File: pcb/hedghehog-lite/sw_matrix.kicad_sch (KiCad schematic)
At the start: 8 parts, among them K00 1u, K01 1u, K10 1u, K11 1u

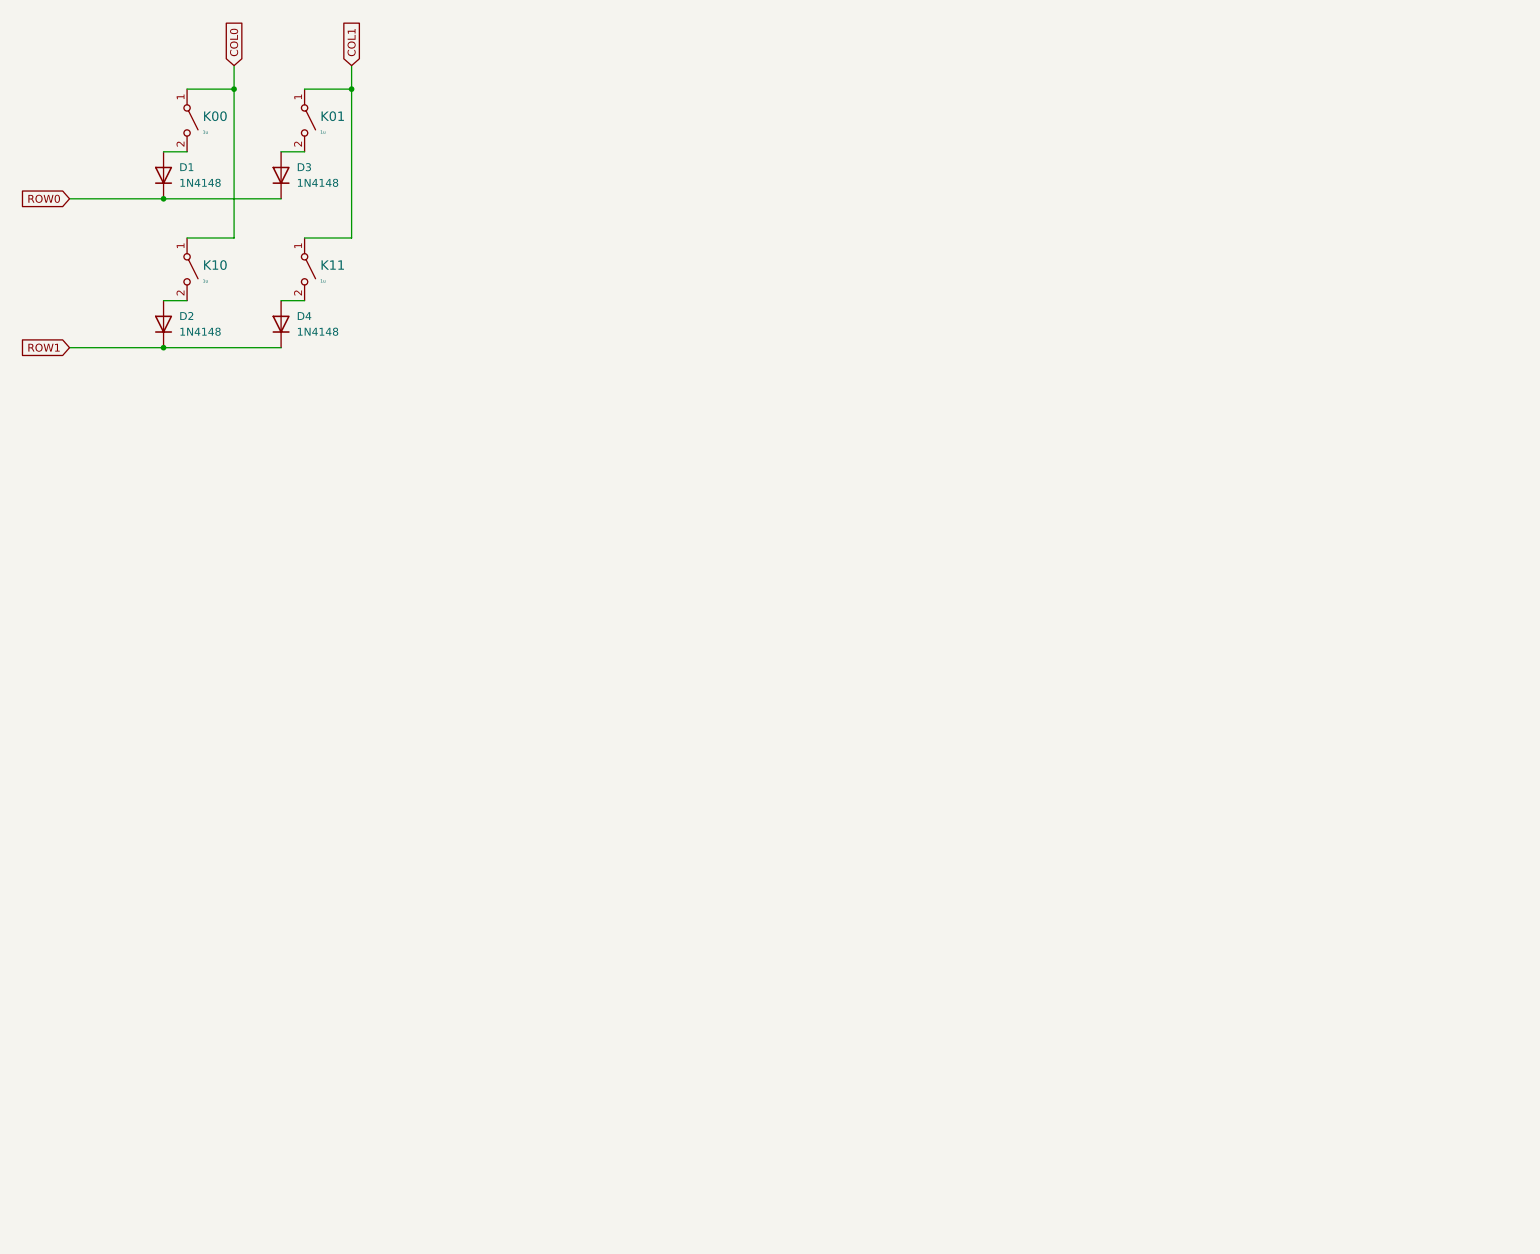
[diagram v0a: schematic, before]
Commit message: More edits to the schematic building v1
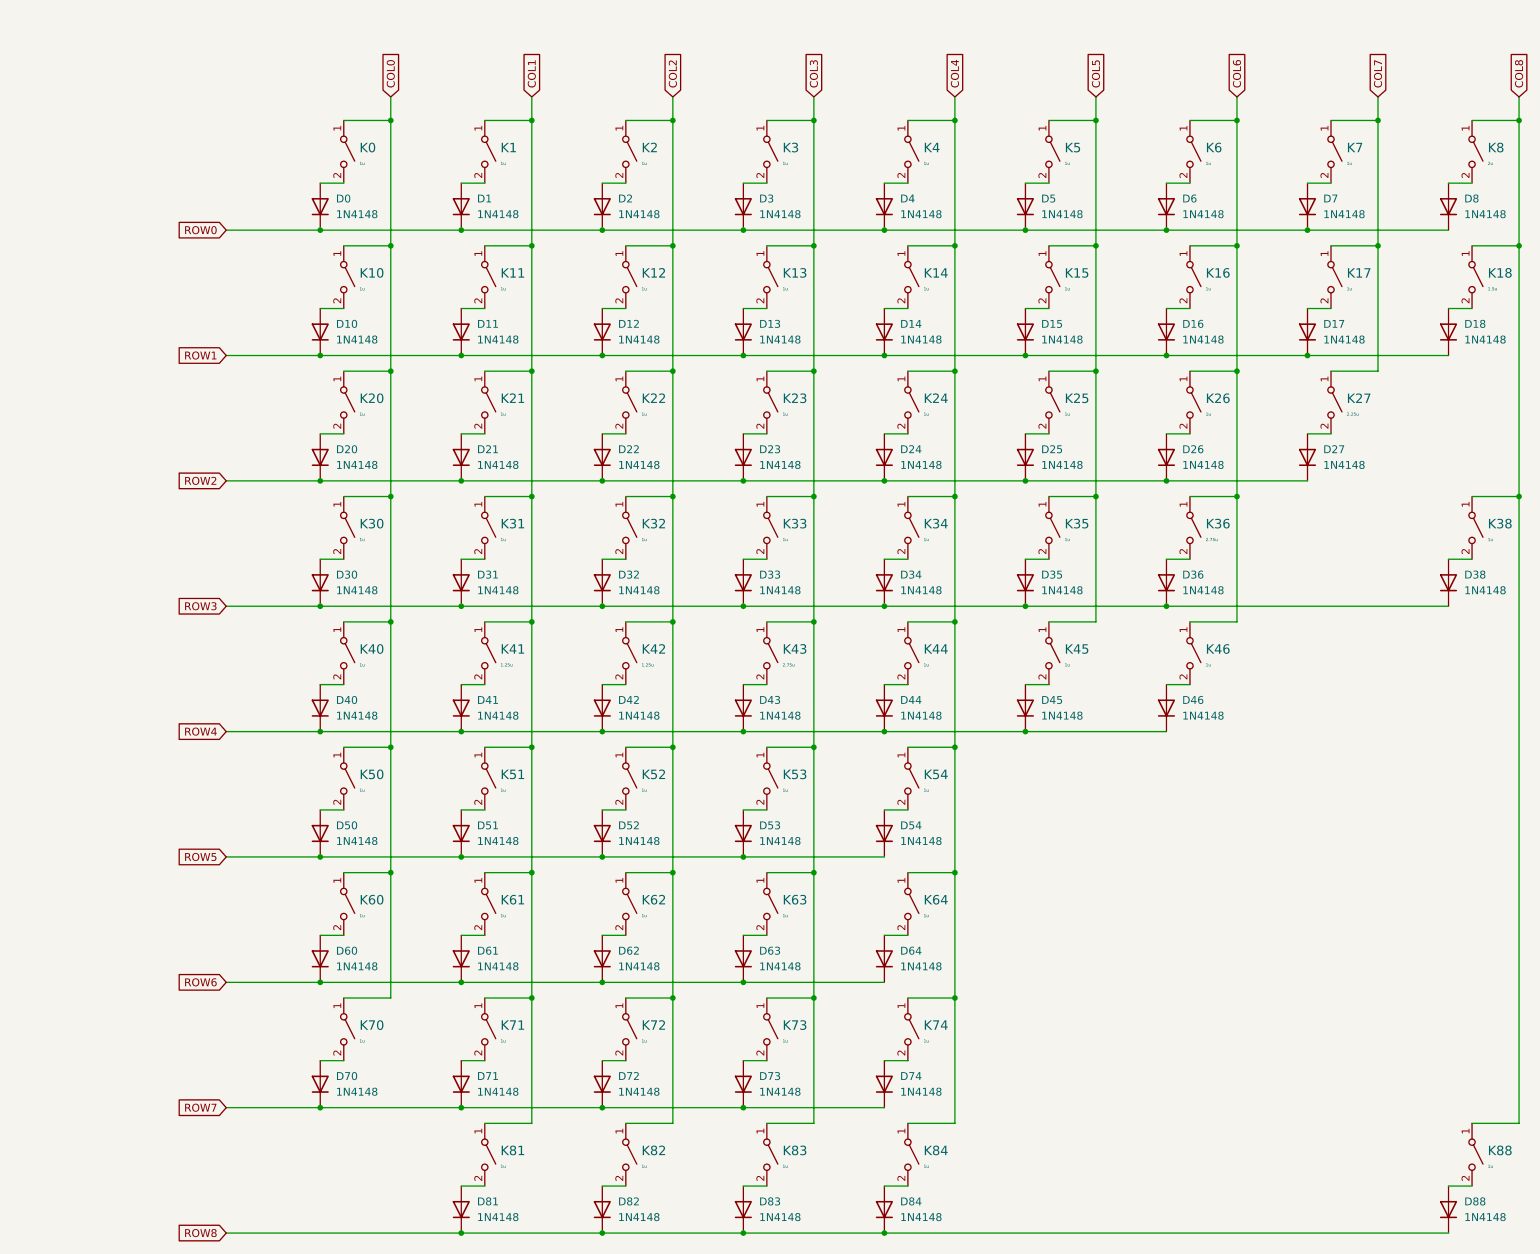
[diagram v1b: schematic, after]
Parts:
- added D12, D13, D14, D15, D16, D17, D18, D2, D3, D4, D5, D6, D7, D70, D8, D81: 1N4148, Diode_SMD:D_0805_2012Metric, symbol Diode:1N4148
- added D20, D21, D22, D23, D24, D25, D26, D27, D30, D31, D32, D33, D34, D35, D36, D38, D40, D41, D42, D43, D44, D45, D46, D50, D51, D52, D53, D54, D60, D61, D62, D63, D64, D71, D72, D73, D74, D82, D83, D84, D88: 1N4148, Diode_THT:D_DO-35_SOD27_P7.62mm_Horizontal, symbol Diode:1N4148
- added K12, K13, K14, K15, K16, K17, K2, K20, K21, K22, K23, K24, K25, K26, K3, K30, K31, K32, K33, K34, K35, K38, K4, K40, K44, K45, K46, K5, K50, K51, K52, K53, K54, K6, K60, K61, K62, K63, K64, K7, K70, K71, K72, K73, K74, K81, K82, K83, K84, K88: 1u, acheron:MX100H, symbol Switch:SW_SPST
- added K18: 1.5u, acheron:MX150H, symbol Switch:SW_SPST
- added K27: 2.25u, acheron:MX225H, symbol Switch:SW_SPST
- added K36: 2.75u, acheron:MX275H, symbol Switch:SW_SPST
- added K41, K42: 1.25u, acheron:MX125H, symbol Switch:SW_SPST
- added K43: 2.75u, acheron:MX275HR, symbol Switch:SW_SPST
- added K8: 2u, acheron:MX200H, symbol Switch:SW_SPST
- D0: renamed from D1; footprint Diode_THT:D_DO-35_SOD27_P7.62mm_Horizontal -> Diode_SMD:D_SOD-123F
- D1: renamed from D3; footprint Diode_THT:D_DO-35_SOD27_P7.62mm_Horizontal -> Diode_SMD:D_0805_2012Metric
- D10: renamed from D2; footprint Diode_THT:D_DO-35_SOD27_P7.62mm_Horizontal -> Diode_SMD:D_0805_2012Metric
- D11: renamed from D4; footprint Diode_THT:D_DO-35_SOD27_P7.62mm_Horizontal -> Diode_SMD:D_0805_2012Metric
- renumbered K00 to K0, K01 to K1
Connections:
- net COL0: now also K20.1 (A), K30.1 (A), K40.1 (A), K50.1 (A), K60.1 (A), K70.1 (A)
- net COL1: now also K21.1 (A), K31.1 (A), K41.1 (A), K51.1 (A), K61.1 (A), K71.1 (A), K81.1 (A)
- net ROW0: now also D2.1 (K), D3.1 (K), D4.1 (K), D5.1 (K), D6.1 (K), D7.1 (K), D8.1 (K)
- net ROW1: now also D12.1 (K), D13.1 (K), D14.1 (K), D15.1 (K), D16.1 (K), D17.1 (K), D18.1 (K)
- new net: D16.2 (A), K16.2 (B)
- new net: D72.2 (A), K72.2 (B)
- new net: D26.2 (A), K26.2 (B)
- new net: D31.2 (A), K31.2 (B)
- new net: D4.2 (A), K4.2 (B)
- new net: D64.2 (A), K64.2 (B)
- new net: D34.2 (A), K34.2 (B)
- new net: D61.2 (A), K61.2 (B)
- new net: D46.2 (A), K46.2 (B)
- new net: D2.2 (A), K2.2 (B)
- new net: D35.2 (A), K35.2 (B)
- new net: D70.2 (A), K70.2 (B)
- new net: D6.2 (A), K6.2 (B)
- new net: D15.2 (A), K15.2 (B)
- new net: D73.2 (A), K73.2 (B)
- new net: D74.2 (A), K74.2 (B)
- new net: D27.2 (A), K27.2 (B)
- new net: D45.2 (A), K45.2 (B)
- new net: D84.2 (A), K84.2 (B)
- new net: D52.2 (A), K52.2 (B)
- new net: D14.2 (A), K14.2 (B)
- new net: D32.2 (A), K32.2 (B)
- new net: D5.2 (A), K5.2 (B)
- new net: D40.2 (A), K40.2 (B)
- new net: D33.2 (A), K33.2 (B)
- new net: D18.2 (A), K18.2 (B)
- new net: D82.2 (A), K82.2 (B)
- new net: D8.2 (A), K8.2 (B)
- new net: D88.2 (A), K88.2 (B)
- new net: D21.2 (A), K21.2 (B)
- new net: D41.2 (A), K41.2 (B)
- new net: D30.2 (A), K30.2 (B)
- new net: D53.2 (A), K53.2 (B)
- new net: D36.2 (A), K36.2 (B)
- new net: D13.2 (A), K13.2 (B)
- new net: D3.2 (A), K3.2 (B)
- new net: D38.2 (A), K38.2 (B)
- new net: D50.2 (A), K50.2 (B)
- new net: D12.2 (A), K12.2 (B)
- new net: D42.2 (A), K42.2 (B)
- new net: D20.2 (A), K20.2 (B)
- new net: D7.2 (A), K7.2 (B)
- new net: D63.2 (A), K63.2 (B)
- new net: D54.2 (A), K54.2 (B)
- new net: D83.2 (A), K83.2 (B)
- new net: D23.2 (A), K23.2 (B)
- new net: D43.2 (A), K43.2 (B)
- new net: D51.2 (A), K51.2 (B)
- new net: D22.2 (A), K22.2 (B)
- new net: D60.2 (A), K60.2 (B)
- new net: D81.2 (A), K81.2 (B)
- new net: D17.2 (A), K17.2 (B)
- new net: D71.2 (A), K71.2 (B)
- new net: D25.2 (A), K25.2 (B)
- new net: D62.2 (A), K62.2 (B)
- new net: D24.2 (A), K24.2 (B)
- new net: D44.2 (A), K44.2 (B)
- new net COL2: K12.1 (A), K2.1 (A), K22.1 (A), K32.1 (A), K42.1 (A), K52.1 (A), K62.1 (A), K72.1 (A), K82.1 (A)
- new net COL3: K13.1 (A), K23.1 (A), K3.1 (A), K33.1 (A), K43.1 (A), K53.1 (A), K63.1 (A), K73.1 (A), K83.1 (A)
- new net COL4: K14.1 (A), K24.1 (A), K34.1 (A), K4.1 (A), K44.1 (A), K54.1 (A), K64.1 (A), K74.1 (A), K84.1 (A)
- new net COL5: K15.1 (A), K25.1 (A), K35.1 (A), K45.1 (A), K5.1 (A)
- new net COL6: K16.1 (A), K26.1 (A), K36.1 (A), K46.1 (A), K6.1 (A)
- new net COL7: K17.1 (A), K27.1 (A), K7.1 (A)
- new net COL8: K18.1 (A), K38.1 (A), K8.1 (A), K88.1 (A)
- new net ROW2: D20.1 (K), D21.1 (K), D22.1 (K), D23.1 (K), D24.1 (K), D25.1 (K), D26.1 (K), D27.1 (K)
- new net ROW3: D30.1 (K), D31.1 (K), D32.1 (K), D33.1 (K), D34.1 (K), D35.1 (K), D36.1 (K), D38.1 (K)
- new net ROW4: D40.1 (K), D41.1 (K), D42.1 (K), D43.1 (K), D44.1 (K), D45.1 (K), D46.1 (K)
- new net ROW5: D50.1 (K), D51.1 (K), D52.1 (K), D53.1 (K), D54.1 (K)
- new net ROW6: D60.1 (K), D61.1 (K), D62.1 (K), D63.1 (K), D64.1 (K)
- new net ROW7: D70.1 (K), D71.1 (K), D72.1 (K), D73.1 (K), D74.1 (K)
- new net ROW8: D81.1 (K), D82.1 (K), D83.1 (K), D84.1 (K), D88.1 (K)
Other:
- moved on the sheet: D0, D1, D10, D11, K0, K1, K10, K11
